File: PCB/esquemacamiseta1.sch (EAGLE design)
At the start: 13 parts, among them IC1 DS18B20

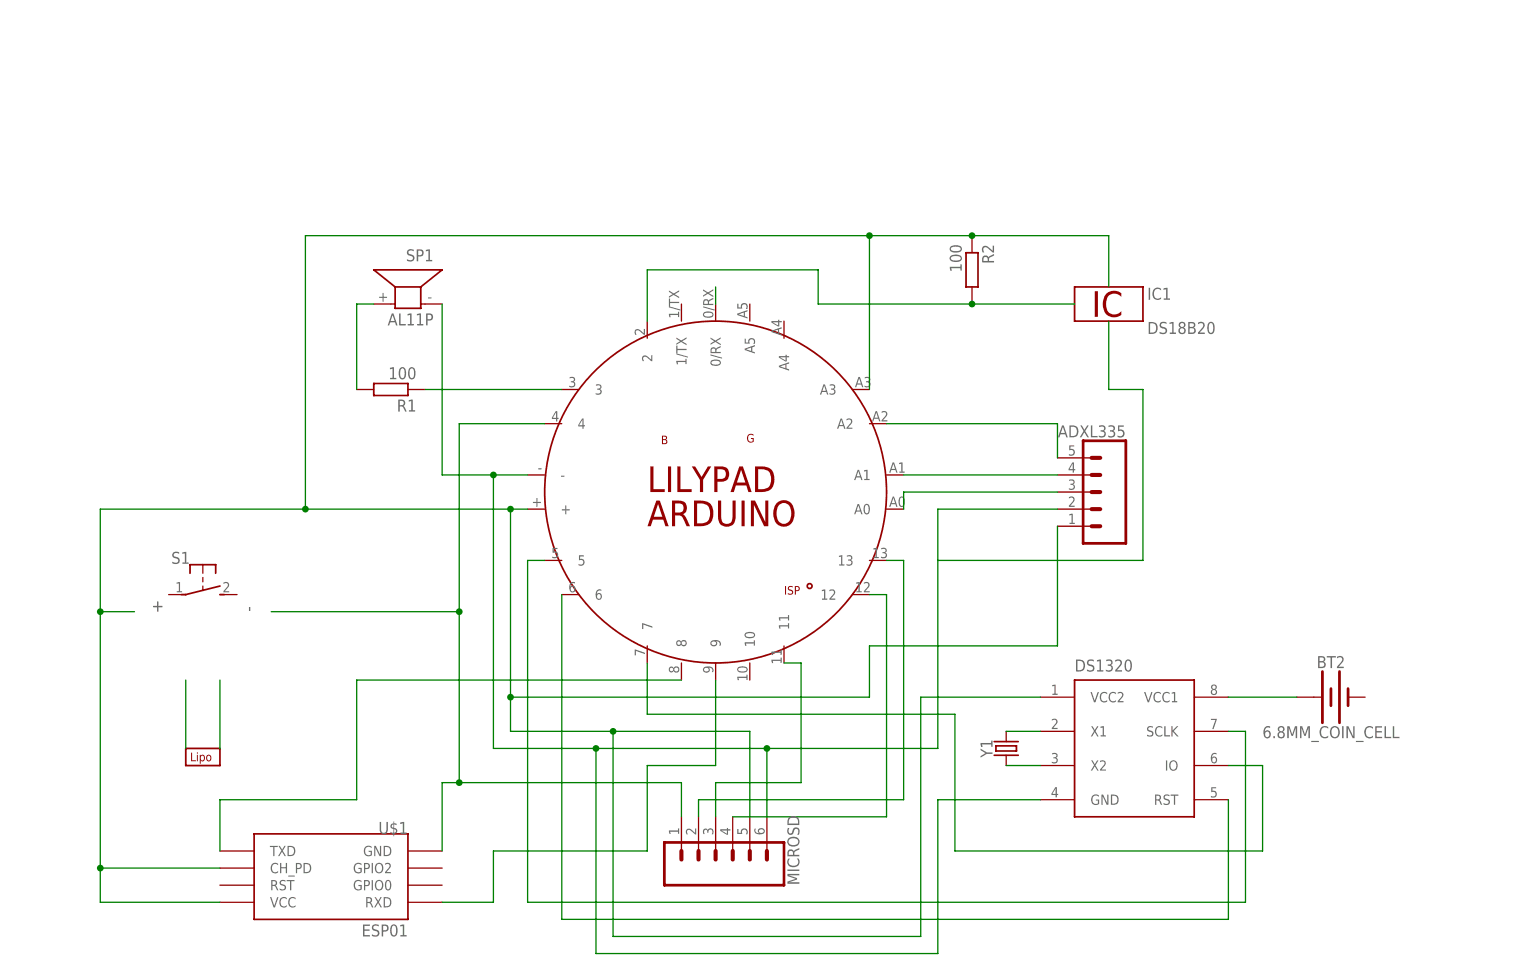
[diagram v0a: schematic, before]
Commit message: Cambios Finales PCB
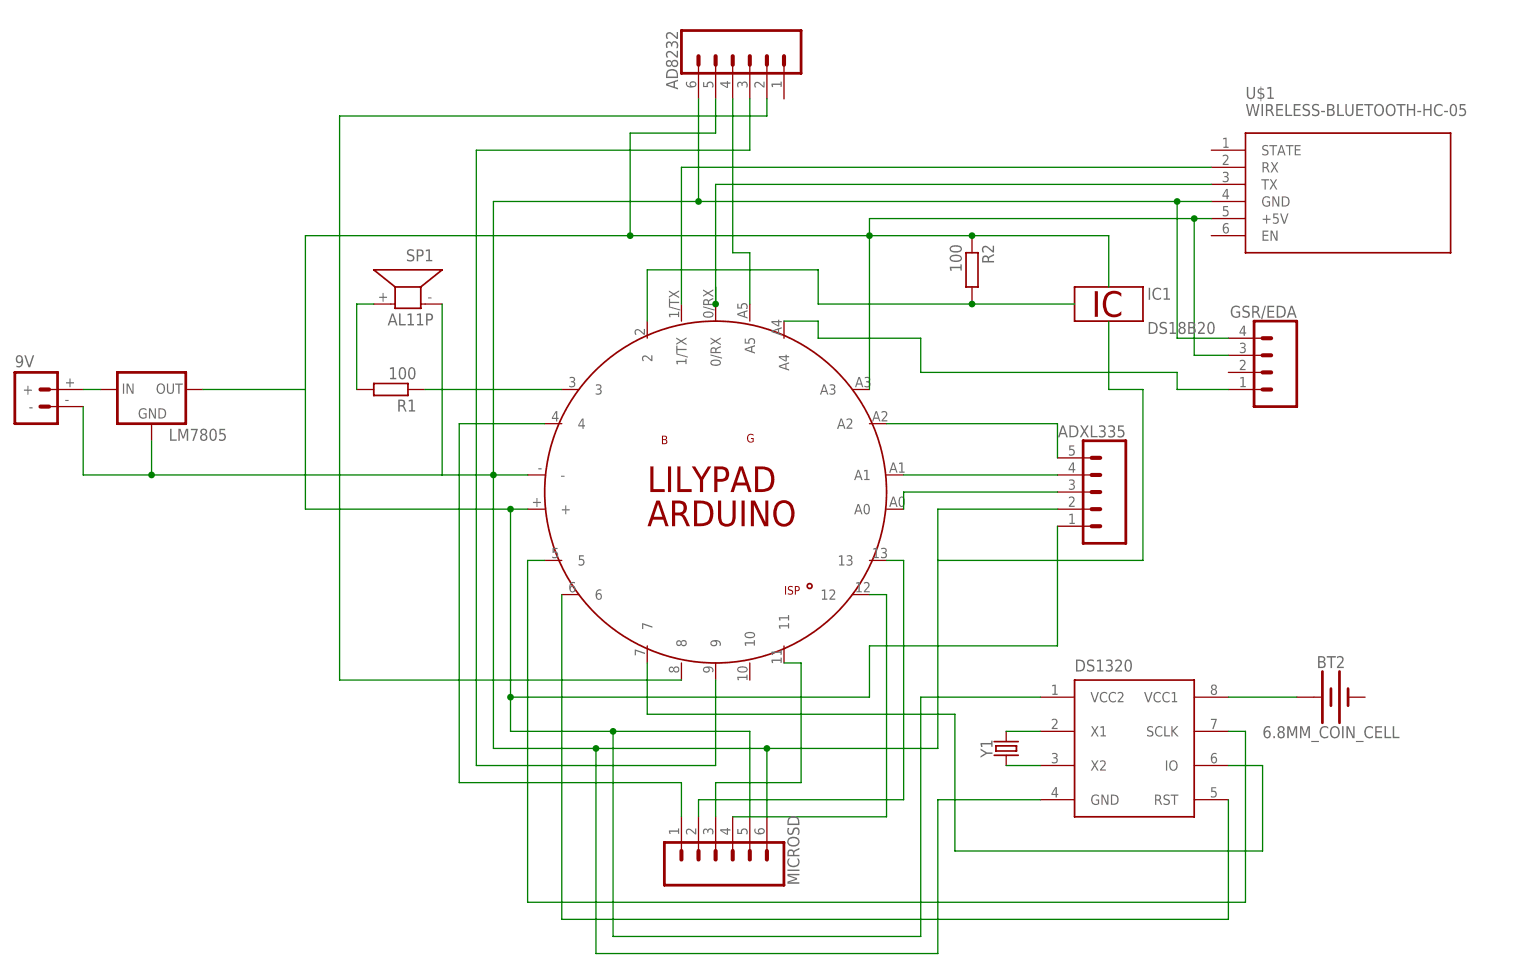
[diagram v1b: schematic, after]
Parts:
- removed BT1: LIPO-OUTLINE1100, SparkFun-Batteries:LIPO-OUTLINE1100
- removed S1: (no value), switch-omron:31-XX
- added 9V: (no value), SparkFun-Connectors:BATTERY_CONN_DEANS
- added AD8232: (no value), SparkFun-Connectors:CONN_06FEMALE_LOCK
- added GSR/EDA: (no value), SparkFun-Connectors:CONN_04JST-PTH
- added LM7805: (no value), SparkFun-IC-Power:V_REG_78XX-TO-220
- U$1: value ESP01 -> WIRELESS-BLUETOOTH-HC-05; device esp8266:ESP01 -> diy-modules:WIRELESS-BLUETOOTH-HC-05
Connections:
- new net N$2: LM7805.OUT
- new net N$24: AD8232.2, PCB1.8
- new net N$25: AD8232.4, PCB1.A5
- new net N$26: AD8232.3, PCB1.9
- new net N$6: 9V.-, AD8232.6, ADXL335.2, DS1320.GND, GSR/EDA.4, LM7805.GND, MICROSD.6, PCB1.-, SP1.1, U$1.GND
- net N$1: no longer U$1.GND
- net N$14: now also U$1.TX
- net N$17: now also 9V.+, LM7805.IN; no longer PCB1.8, U$1.TXD
- net N$19: now also GSR/EDA.1, PCB1.A4; no longer PCB1.9, U$1.RXD
- net N$3: now also AD8232.5, GSR/EDA.3, U$1.+5V; no longer U$1.CH_PD, U$1.VCC
- net N$5: now also PCB1.1/TX, U$1.RX; no longer ADXL335.2, DS1320.GND, MICROSD.6, PCB1.-, SP1.1
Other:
- note removed: "+"
- note removed: "-"
- note removed: "Lilypad Simple Power"

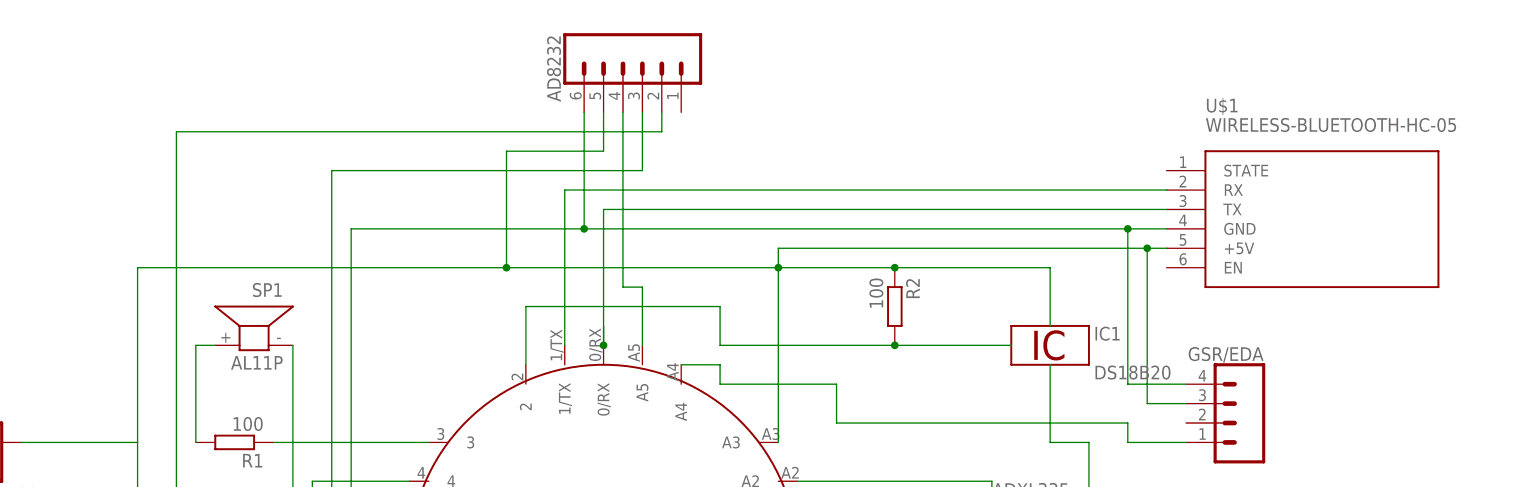
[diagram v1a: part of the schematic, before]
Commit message: Cambios PCB
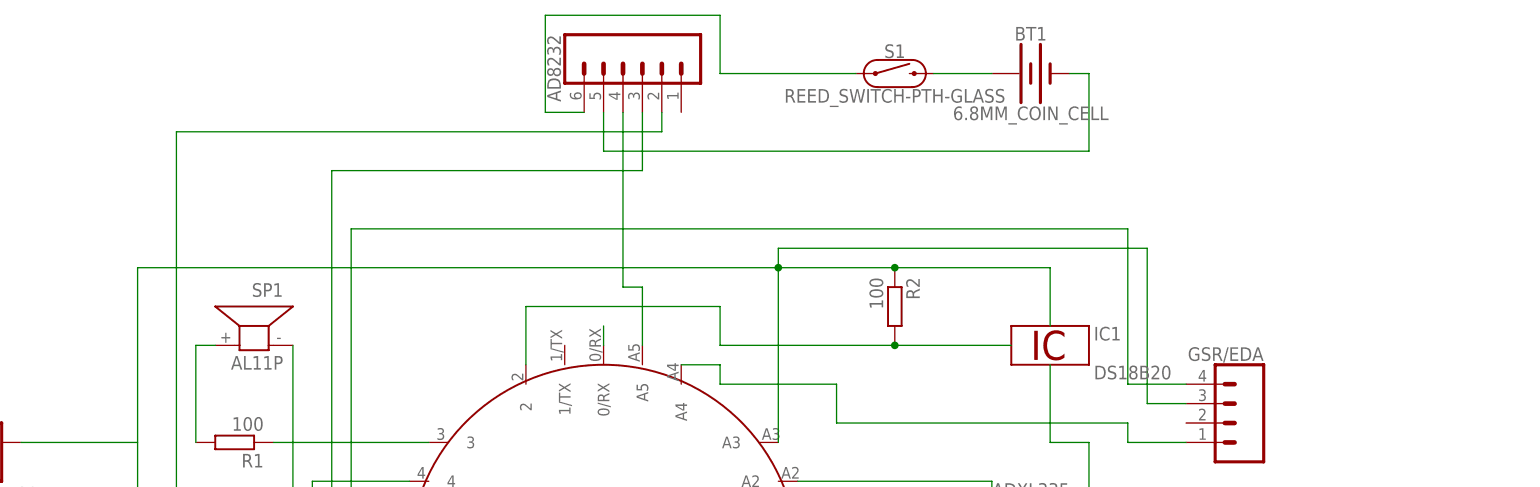
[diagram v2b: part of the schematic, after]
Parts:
- removed U$1: WIRELESS-BLUETOOTH-HC-05, diy-modules:WIRELESS-BLUETOOTH-HC-05
- added BT1: 6.8MM_COIN_CELL, SparkFun-Batteries:BATTERY-6.8MM_SMD
- added S1: REED_SWITCH-PTH-GLASS, SparkFun-Switches:REED_SWITCH-PTH-GLASS
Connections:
- new net N$27: AD8232.6, S1.1
- new net N$28: AD8232.5, BT1.-
- net N$14: now also BT1.+, S1.2; no longer PCB1.0/RX, U$1.TX
- net N$3: no longer AD8232.5, U$1.+5V
- net N$5: now also PCB1.0/RX; no longer PCB1.1/TX, U$1.RX
- net N$6: no longer AD8232.6, U$1.GND
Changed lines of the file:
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@@
 <part name="LM7805" library="SparkFun-IC-Power" deviceset="V_REG_78XX" device="-TO-220"/>
 <part name="9V" library="SparkFun-Connectors" deviceset="BATTERY_CONN" device="_DEANS"/>
-<part name="U$1" library="diy-modules" deviceset="WIRELESS-BLUETOOTH-HC-05" device=""/>
 <part name="GSR/EDA" library="SparkFun-Connectors" deviceset="CONN_04" device="JST-PTH"/>
 <part name="AD8232" library="SparkFun-Connectors" deviceset="CONN_06" device="FEMALE_LOCK"/>
+<part name="S1" library="SparkFun-Switches" deviceset="REED_SWITCH" device="-PTH-GLASS"/>
+<part name="BT1" library="SparkFun-Batteries" deviceset="BATTERY" device="-6.8MM_SMD" value="6.8MM_COIN_CELL"/>
 </parts>
 <sheets>
@@
 <attribute name="NAME" x="-40.64" y="61.722" size="1.778" layer="95" font="vector"/>
 </instance>
-<instance part="U$1" gate="G$1" x="157.48" y="88.9" smashed="yes">
-<attribute name="NAME" x="142.24" y="101.6" size="1.778" layer="95"/>
-<attribute name="VALUE" x="142.24" y="99.06" size="1.778" layer="96"/>
-</instance>
 <instance part="GSR/EDA" gate="J1" x="144.78" y="60.96" smashed="yes" rot="MR0">
 <attribute name="VALUE" x="149.86" y="53.594" size="1.778" layer="96" font="vector" rot="MR0"/>
@@
 <attribute name="VALUE" x="78.486" y="111.76" size="1.778" layer="96" font="vector" rot="MR270"/>
 <attribute name="NAME" x="57.912" y="111.76" size="1.778" layer="95" font="vector" rot="MR270"/>
+</instance>
+<instance part="S1" gate="G$1" x="101.6" y="106.68" smashed="yes">
+<attribute name="NAME" x="101.6" y="108.712" size="1.778" layer="95" font="vector" align="bottom-center"/>
+<attribute name="VALUE" x="101.6" y="104.648" size="1.778" layer="96" font="vector" align="top-center"/>
+</instance>
+<instance part="BT1" gate="G$1" x="119.38" y="106.68" smashed="yes">
+<attribute name="NAME" x="119.38" y="110.998" size="1.778" layer="95" font="vector" align="bottom-center"/>
+<attribute name="VALUE" x="119.38" y="102.362" size="1.778" layer="96" font="vector" align="top-center"/>
 </instance>
 </instances>
@@
 </busses>
 <nets>
-<net name="N$14" class="0">
-<segment>
-<pinref part="PCB1" gate="G$1" pin="0/RX"/>
-<wire x1="63.5" y1="73.66" x2="63.5" y2="71.12" width="0.1524" layer="91"/>
-<wire x1="63.5" y1="71.12" x2="63.5" y2="88.9" width="0.1524" layer="91"/>
-<junction x="63.5" y="71.12"/>
-<pinref part="U$1" gate="G$1" pin="TX"/>
-<wire x1="63.5" y1="88.9" x2="137.16" y2="88.9" width="0.1524" layer="91"/>
-</segment>
-</net>
 <net name="N$18" class="0">
 <segment>
@@
 <wire x1="2.54" y1="40.64" x2="2.54" y2="81.28" width="0.1524" layer="91"/>
 <pinref part="PCB1" gate="G$1" pin="A3"/>
-<wire x1="2.54" y1="81.28" x2="50.8" y2="81.28" width="0.1524" layer="91"/>
-<wire x1="50.8" y1="81.28" x2="86.36" y2="81.28" width="0.1524" layer="91"/>
+<wire x1="2.54" y1="81.28" x2="86.36" y2="81.28" width="0.1524" layer="91"/>
 <wire x1="86.36" y1="81.28" x2="86.36" y2="58.42" width="0.1524" layer="91"/>
 <pinref part="DS1320" gate="G$1" pin="VCC2"/>
@@
 <pinref part="R2" gate="G$1" pin="1"/>
 <junction x="101.6" y="81.28"/>
-<pinref part="U$1" gate="G$1" pin="+5V"/>
-<wire x1="137.16" y1="83.82" x2="134.62" y2="83.82" width="0.1524" layer="91"/>
 <wire x1="134.62" y1="83.82" x2="86.36" y2="83.82" width="0.1524" layer="91"/>
 <wire x1="86.36" y1="83.82" x2="86.36" y2="81.28" width="0.1524" layer="91"/>
@@
 <wire x1="139.7" y1="63.5" x2="134.62" y2="63.5" width="0.1524" layer="91"/>
 <wire x1="134.62" y1="63.5" x2="134.62" y2="83.82" width="0.1524" layer="91"/>
-<junction x="134.62" y="83.82"/>
-<pinref part="AD8232" gate="G$1" pin="5"/>
-<wire x1="63.5" y1="101.6" x2="63.5" y2="96.52" width="0.1524" layer="91"/>
-<wire x1="63.5" y1="96.52" x2="50.8" y2="96.52" width="0.1524" layer="91"/>
-<wire x1="50.8" y1="96.52" x2="50.8" y2="81.28" width="0.1524" layer="91"/>
-<junction x="50.8" y="81.28"/>
 </segment>
 </net>
@@
 <wire x1="121.92" y1="58.42" x2="121.92" y2="68.58" width="0.1524" layer="91"/>
 <wire x1="30.48" y1="45.72" x2="30.48" y2="86.36" width="0.1524" layer="91"/>
-<pinref part="U$1" gate="G$1" pin="GND"/>
-<wire x1="30.48" y1="86.36" x2="60.96" y2="86.36" width="0.1524" layer="91"/>
-<wire x1="60.96" y1="86.36" x2="132.08" y2="86.36" width="0.1524" layer="91"/>
-<wire x1="132.08" y1="86.36" x2="137.16" y2="86.36" width="0.1524" layer="91"/>
+<wire x1="30.48" y1="86.36" x2="132.08" y2="86.36" width="0.1524" layer="91"/>
 <wire x1="132.08" y1="86.36" x2="132.08" y2="66.04" width="0.1524" layer="91"/>
-<junction x="132.08" y="86.36"/>
 <pinref part="GSR/EDA" gate="J1" pin="4"/>
 <wire x1="132.08" y1="66.04" x2="139.7" y2="66.04" width="0.1524" layer="91"/>
-<pinref part="AD8232" gate="G$1" pin="6"/>
-<wire x1="60.96" y1="101.6" x2="60.96" y2="86.36" width="0.1524" layer="91"/>
-<junction x="60.96" y="86.36"/>
 </segment>
 </net>
@@
 <pinref part="LM7805" gate="G$1" pin="IN"/>
 <wire x1="-30.48" y1="58.42" x2="-27.94" y2="58.42" width="0.1524" layer="91"/>
-</segment>
-</net>
-<net name="N$5" class="0">
-<segment>
-<pinref part="U$1" gate="G$1" pin="RX"/>
-<wire x1="137.16" y1="91.44" x2="58.42" y2="91.44" width="0.1524" layer="91"/>
-<pinref part="PCB1" gate="G$1" pin="1/TX"/>
-<wire x1="58.42" y1="91.44" x2="58.42" y2="71.12" width="0.1524" layer="91"/>
 </segment>
 </net>
@@
 </segment>
 </net>
+<net name="N$5" class="0">
+<segment>
+<pinref part="PCB1" gate="G$1" pin="0/RX"/>
+<wire x1="63.5" y1="73.66" x2="63.5" y2="71.12" width="0.1524" layer="91"/>
+</segment>
+</net>
+<net name="N$14" class="0">
+<segment>
+<pinref part="BT1" gate="G$1" pin="+"/>
+<pinref part="S1" gate="G$1" pin="2"/>
+<wire x1="114.3" y1="106.68" x2="106.68" y2="106.68" width="0.1524" layer="91"/>
+</segment>
+</net>
+<net name="N$27" class="0">
+<segment>
+<pinref part="S1" gate="G$1" pin="1"/>
+<wire x1="96.52" y1="106.68" x2="78.74" y2="106.68" width="0.1524" layer="91"/>
+<wire x1="78.74" y1="106.68" x2="78.74" y2="114.3" width="0.1524" layer="91"/>
+<wire x1="78.74" y1="114.3" x2="55.88" y2="114.3" width="0.1524" layer="91"/>
+<wire x1="55.88" y1="114.3" x2="55.88" y2="101.6" width="0.1524" layer="91"/>
+<pinref part="AD8232" gate="G$1" pin="6"/>
+<wire x1="55.88" y1="101.6" x2="60.96" y2="101.6" width="0.1524" layer="91"/>
+</segment>
+</net>
+<net name="N$28" class="0">
+<segment>
+<pinref part="AD8232" gate="G$1" pin="5"/>
+<wire x1="63.5" y1="101.6" x2="63.5" y2="96.52" width="0.1524" layer="91"/>
+<wire x1="63.5" y1="96.52" x2="127" y2="96.52" width="0.1524" layer="91"/>
+<wire x1="127" y1="96.52" x2="127" y2="106.68" width="0.1524" layer="91"/>
+<pinref part="BT1" gate="G$1" pin="-"/>
+<wire x1="127" y1="106.68" x2="124.46" y2="106.68" width="0.1524" layer="91"/>
+</segment>
+</net>
